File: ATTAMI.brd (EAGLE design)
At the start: 27.9 x 46.7 mm, 27 parts, among them Q1 NTD3055L, Q2 NTD3055L, Q3 NTD3055L, SW1 SPST_TACT-KMR2, U1 NCP4626 (5V), U2 ATTINY85

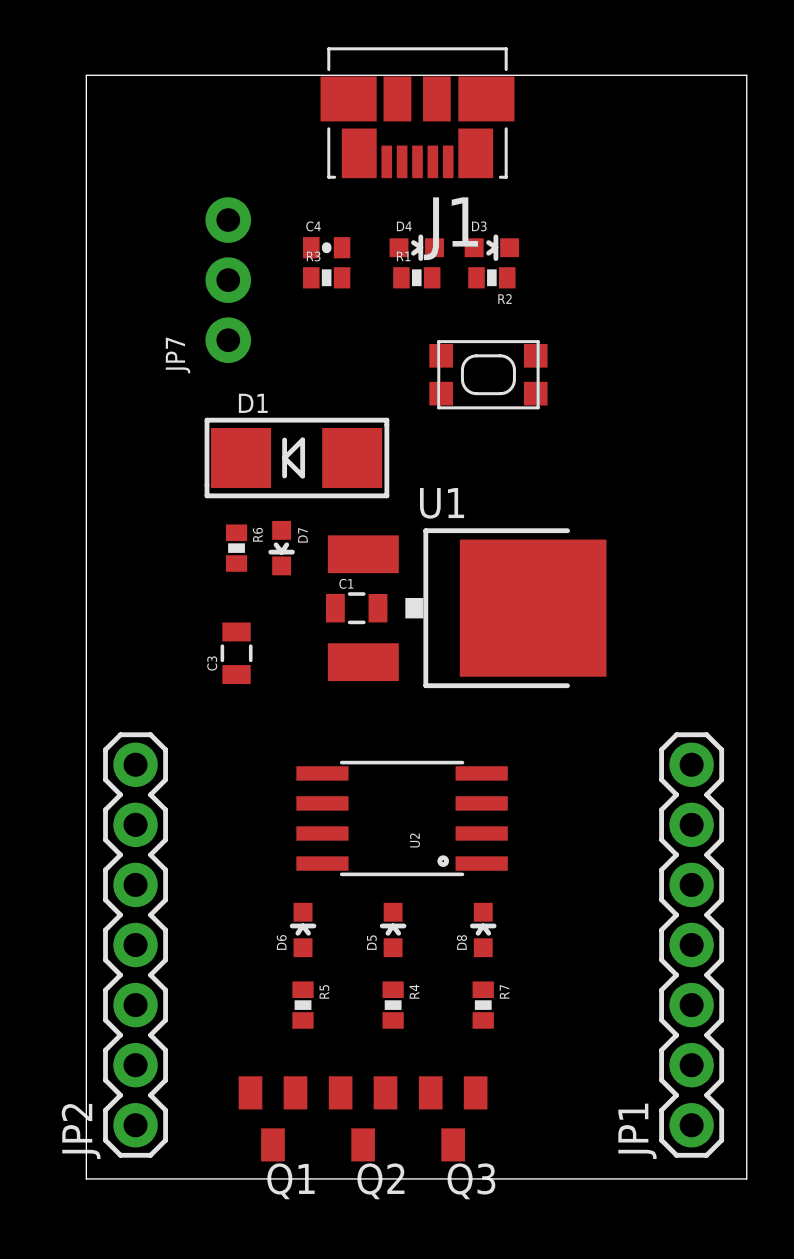
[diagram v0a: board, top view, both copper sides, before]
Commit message: ver07
http://i.imgur.com/BFdtqUi.jpg
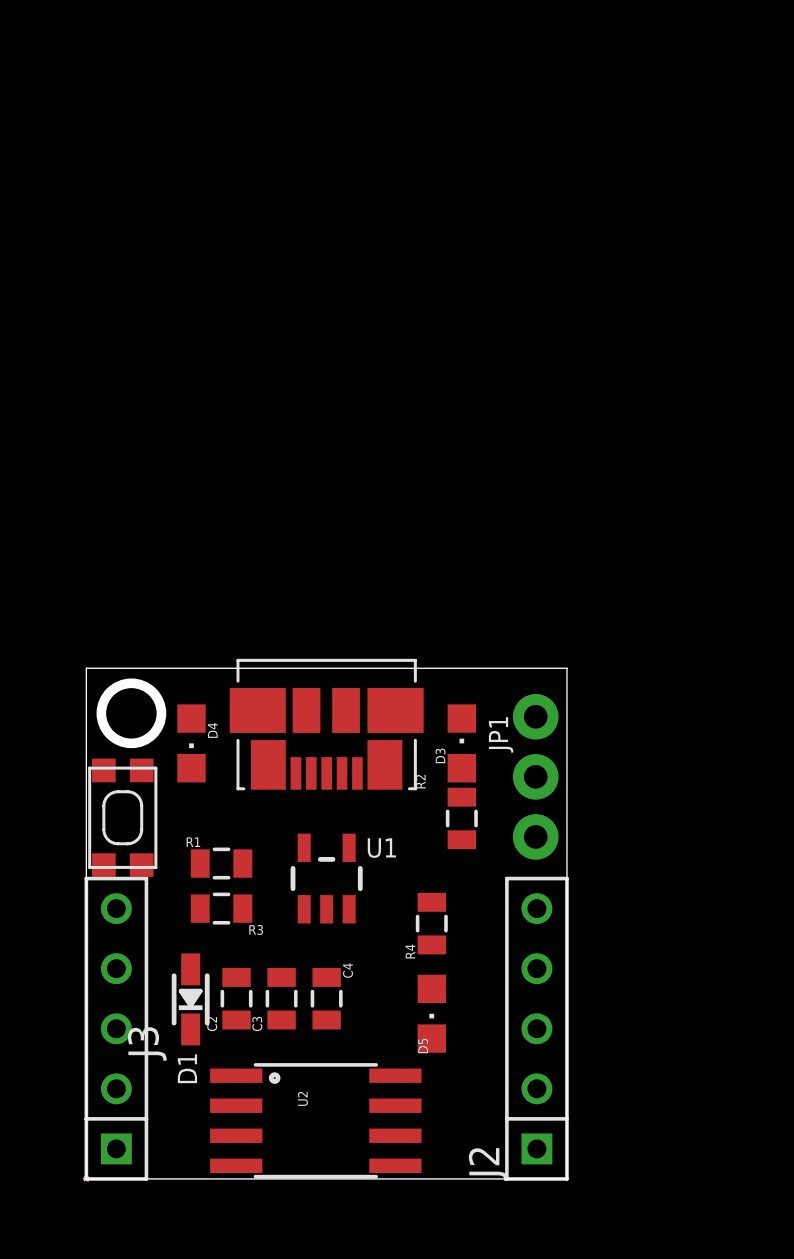
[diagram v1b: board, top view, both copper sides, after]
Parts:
- removed C1: 4.7uf, SparkFun:0805
- removed D6: Red LED, SparkFun:LED-0603
- removed D7: Green LED, SparkFun:LED-0603
- removed D8: Blue LED, SparkFun:LED-0603
- removed JP2: (no value), SparkFun:1X07
- removed JP7: (no value), microbuilder:1X03_ROUND_76
- removed Q1, Q2, Q3: NTD3055L, transistor-small-signal:SOT23
- removed R5: 560R, SparkFun:0402-RES
- removed R6, R7: 330R, SparkFun:0402-RES
- added C2: 4.7uf, SparkFun:0805
- added J2, J3: CON_HEADER_1X05-PTH, dp_devices:M1X5
- C4: device SparkFun:0402-CAP -> SparkFun:0805
- D1: device microbuilder:SMADIODE -> microbuilder:SOD-323
- D3, D4, D5: device SparkFun:LED-0603 -> dp_devices:LED-805
- JP1: device SparkFun:1X07 -> microbuilder:1X03_ROUND_76
- R1, R2, R3, R4: device SparkFun:0402-RES -> SparkFun:0805
- U1: value NCP4626 (5V) -> NCP4626; device v-reg:DPACK -> yair_r:SOT23-5
- moved C4 31.7 mm to (10.2, 7.62), turned to 270 degrees
- moved R3 27.0 mm to (5.71, 11.4), turned to 180 degrees
- moved J1 26.1 mm to (10.2, 17.1)
- moved R1 26.1 mm to (5.71, 13.3)
- moved SW1 24.3 mm to (1.54, 15.3), turned to 270 degrees
- moved D1 23.3 mm to (4.41, 7.59), turned to 90 degrees
- moved D4 23.0 mm to (4.45, 18.4), turned to 180 degrees
- moved R2 22.9 mm to (15.9, 15.2), turned to 270 degrees
- moved D3 21.0 mm to (15.9, 18.4), turned to 0 degrees
- moved JP1 16.1 mm to (19.0, 17.0), turned to 270 degrees
- moved C3 14.7 mm to (8.26, 7.62)
- moved U2 13.3 mm to (9.71, 2.46), turned to 270 degrees
- moved U1 13.1 mm to (10.2, 12.7), turned to 0 degrees
- moved D5 3.90 mm to (14.6, 6.99), turned to 180 degrees
- moved R4 3.81 mm to (14.6, 10.8), turned to 90 degrees
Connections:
- removed net N$12: D7.A, R6.1
- removed net N$13: D6.A, R5.1
- removed net N$14: D8.A, R7.1
- removed net N$16: JP2.3, Q3.3
- removed net N$4: JP2.2, Q2.3
- removed net N$9: JP2.1, Q1.3
- net GND: now also C2.2, J2.5, J3.5, JP1.1, JP1.3, U1.2; no longer C1.2, D6.C, D7.C, D8.C, JP1.7, JP2.4, JP2.6, JP7.1, JP7.3, Q1.2, Q2.2, Q3.2, U1.4
- net N$1: now also J3.1; no longer JP1.4
- net N$15: now also J2.2; no longer JP1.2, Q2.1, R6.2
- net N$3: now also J2.1; no longer JP1.1, Q1.1, R5.2
- net N$5: now also J2.3; no longer JP1.3, Q3.1, R7.2
- net N$6: now also J3.2; no longer JP1.5
- net N$8: now also J3.3; no longer JP1.6
- net VCC: now also J2.4, U1.4; no longer JP2.5, U1.3
- net V_BAT: now also C2.1, J3.4, JP1.2, U1.3, U1.5; no longer C1.1, JP7.2
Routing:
- net N$2: track 0.00 -> 0.85 mm
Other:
- board size 27.9 x 46.7 mm -> 20.3 x 21.6 mm
